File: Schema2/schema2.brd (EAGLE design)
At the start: 53 x 64.8 mm, 34 parts, among them IC1 LM2596S, IC2 78L05CPK, IC3 TL431ACDBZ, IC4 LM358D, X1 22-23-2021, X2 22-23-2021

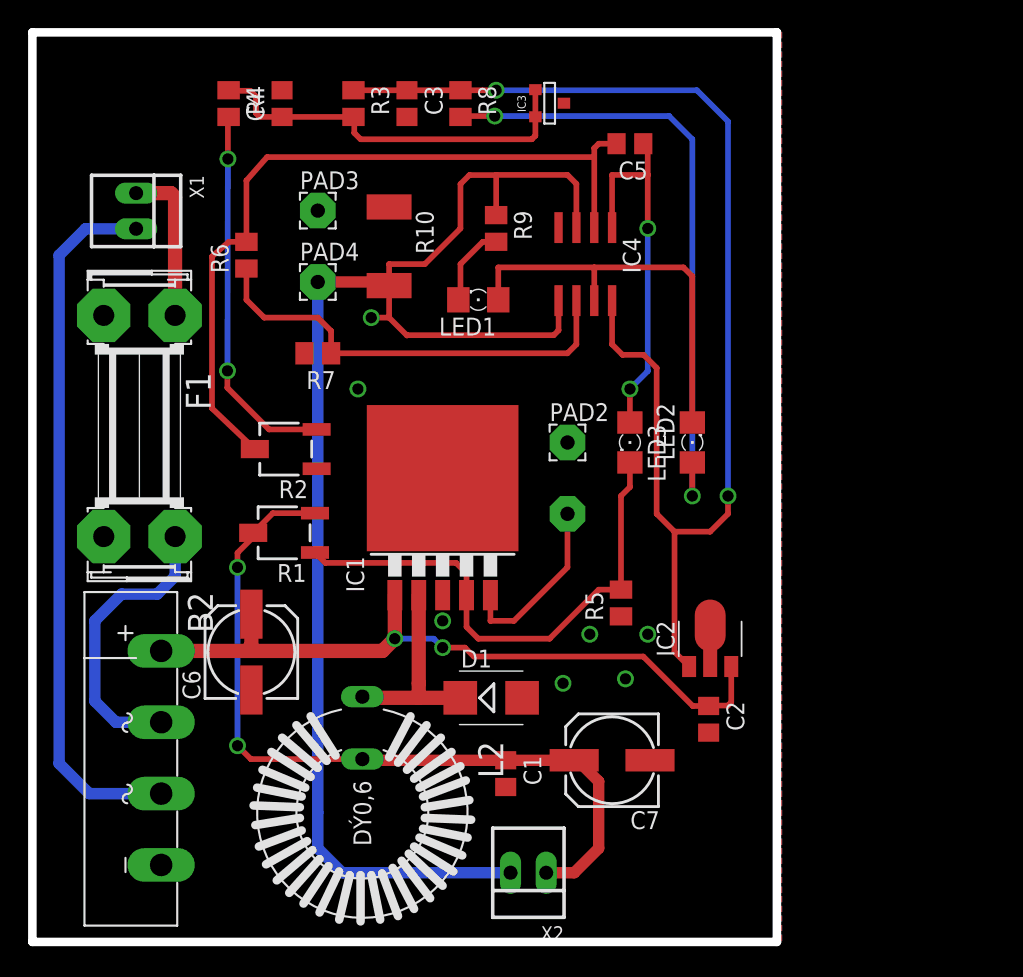
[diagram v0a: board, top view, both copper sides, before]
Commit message: update schema
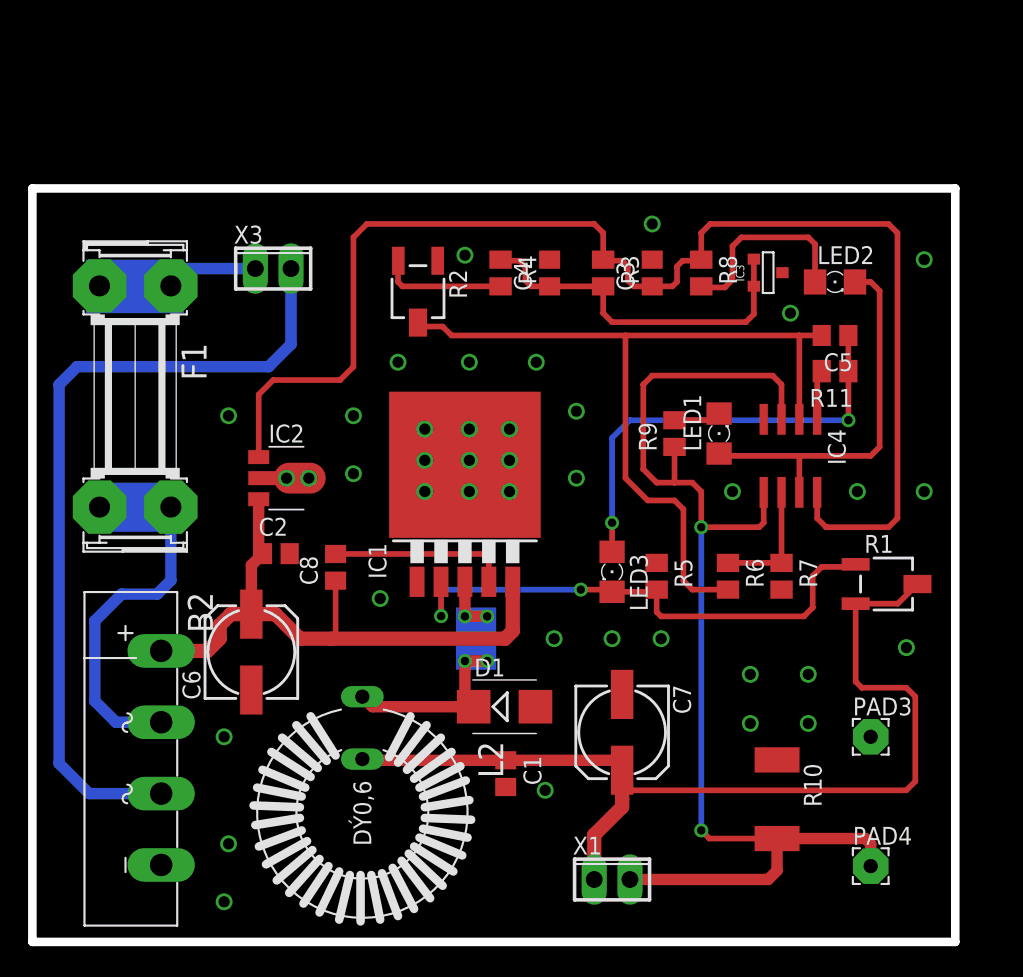
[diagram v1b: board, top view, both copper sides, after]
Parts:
- removed PAD1, PAD2: (no value), wirepad:2,54/1,0
- removed X2: 22-23-2021, con-molex:22-23-2021
- added C8: 1uF, eagle-ltspice:C0805
- added R11: 80R, resistor:M0805
- added X3: (no value), con-phoenix-254:2POL254
- IC1: value LM2596S -> XL4015; device linear:TO263-5 -> moje:TO263-5
- X1: value 22-23-2021 -> (none); device con-molex:22-23-2021 -> con-phoenix-254:2POL254
- moved X1 58.4 mm to (41.3, 4.45), turned to 0 degrees
- moved PAD4 57.3 mm to (59.7, 5.40)
- moved PAD3 54.3 mm to (59.7, 14.6)
- moved R10 48.1 mm to (53.0, 10.2)
- moved R1 43.0 mm to (60.8, 25.5), turned to 0 degrees
- moved R6 41.2 mm to (49.5, 26.0), turned to 270 degrees
- moved R7 36.6 mm to (53.3, 26.0), turned to 270 degrees
- moved C2 33.0 mm to (17.4, 27.6), turned to 0 degrees
- moved IC2 32.3 mm to (18.1, 33.0), turned to 270 degrees
- moved R4 22.8 mm to (33.3, 47.6)
- moved C4 22.5 mm to (36.8, 47.6)
- moved R3 21.5 mm to (40.6, 47.6)
- moved C3 21.2 mm to (44.1, 47.6), turned to 90 degrees
- moved R8 21.0 mm to (47.6, 47.6)
- moved C5 20.0 mm to (57.1, 43.2)
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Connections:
- removed net N$8: IC1.5, PAD1.1
- new net N$4: IC4.1, R11.2
- new net N$5: C8.2, IC1.4
- net GND: now also IC1.1; no longer IC1.3, PAD2.1
- net N$1: now also X3.1; no longer X1.1
- net N$10: now also IC1.3; no longer IC1.2
- net N$11: now also R11.1; no longer IC4.1
- net N$12: now also X1.1; no longer X2.1
- net N$14: now also IC1.2; no longer IC1.4
- net N$21: now also X1.2; no longer X2.2
- net N$3: now also X3.2; no longer X1.2
- net VCC_IN: now also C8.1, IC1.5; no longer IC1.1
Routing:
- net N$20: track 45.0 -> 13.9 mm, vias 2 -> 0
- net N$16: track 31.6 -> 8.83 mm
- net N$21: track 103.9 -> 84.1 mm, vias 1 -> 2
- net N$7: track 27.1 -> 8.95 mm, vias 2 -> 0
- net N$12: track 57.1 -> 70.6 mm, vias 2 -> 0
- net N$8: track 12.7 -> 0.00 mm
- net N$5: track 0.00 -> 12.6 mm
- net N$3: track 50.6 -> 58.2 mm
- net VCC_IN: track 51.5 -> 44.2 mm, vias 2 -> 0
- net N$6: track 89.1 -> 96.2 mm, vias 2 -> 0
- net N$10: track 14.3 -> 20.6 mm, vias 0 -> 4
- net N$1: track 11.3 -> 6.53 mm
- net N$11: track 26.8 -> 31.5 mm
- net N$4: track 0.00 -> 3.75 mm
- net N$9: track 55.1 -> 58.8 mm
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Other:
- board size 53 x 64.8 mm -> 65.7 x 53.6 mm

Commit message: update schema
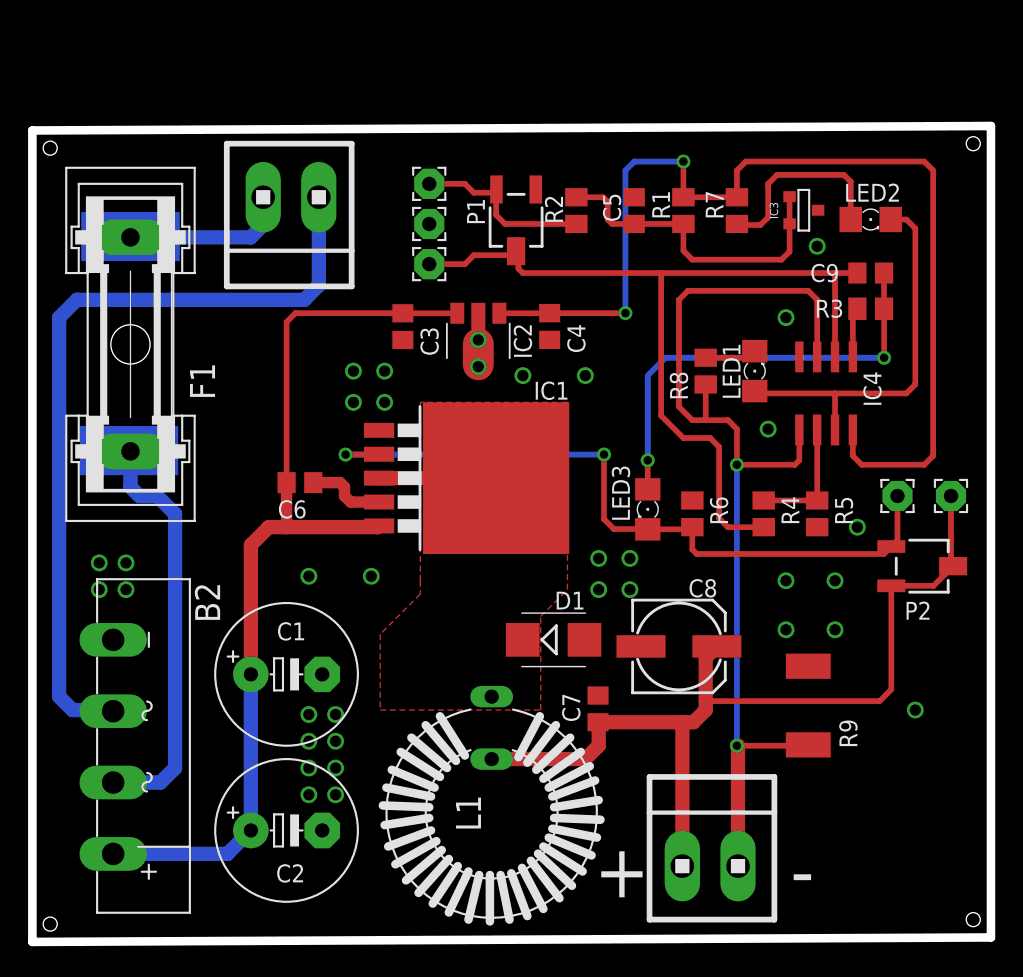
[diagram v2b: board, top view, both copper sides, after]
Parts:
- removed L2: 40uH, inductors:ED16
- removed R10: 0,05R, eagle-ltspice:R2512
- removed R11: 80R, resistor:M0805
- removed X1, X3: (no value), con-phoenix-254:2POL254
- added C9: 1uF, eagle-ltspice:C0805
- added J1, J2: (no value), con-amp:1X2MTA
- added L1: 40uH, inductors:ED16
- added P1, P2: 10K, pot:3223G
- added PAD2, PAD5, PAD6: (no value), wirepad:2,15/1,0
- C1, C2: value 10uF -> (none); device eagle-ltspice:C0805 -> adafruit:E5-10,5
- C3: value 1uF -> 10uF
- C6: value 470uF -> 1uF; device resistor:153CLV-0605 -> eagle-ltspice:C0805
- C7: value 470uF -> 10uF; device resistor:153CLV-0605 -> eagle-ltspice:C0805
- C8: value 1uF -> 470uF; device eagle-ltspice:C0805 -> resistor:153CLV-0605
- F1: value (none) -> FUSEGSH15; device fuse:SHK20Q -> fuse:GSH15
- IC2: value 78L05CPK -> 78L05
- IC3: value TL431ACDBZ -> TL431
- PAD3, PAD4: device wirepad:2,54/1,0 -> wirepad:2,15/1,0
- R1: value 10K -> 2,2K; device pot:3223G -> resistor:M0805
- R2: value 10K -> 68K; device pot:3223G -> resistor:M0805
- R3: value 2,2K -> 80R
- R4: value 71,5K -> 100K
- R5: value 270R -> 10K
- R6: value 90,9K -> 270R
- R7: value 10K -> 1K
- R9: value 1K -> 0,05R; device resistor:M0805 -> eagle-ltspice:R2512
- moved PAD4 57.9 mm to (28.3, 54.0)
- moved R1 30.3 mm to (46.4, 52.1), turned to 270 degrees
- moved R7 26.2 mm to (50.2, 52.1)
- moved R4 25.4 mm to (52.1, 30.5)
- moved C8 25.1 mm to (46.0, 21.0), turned to 0 degrees
- moved R9 21.6 mm to (55.2, 16.8), turned to 270 degrees
- moved C2 19.7 mm to (18.1, 7.94)
- moved R3 19.2 mm to (59.7, 45.1), turned to 180 degrees
- moved C3 18.2 mm to (26.4, 43.8), turned to 270 degrees
- moved PAD3 18.1 mm to (65.4, 31.8)
- moved C1 17.1 mm to (18.1, 19.1), turned to 0 degrees
- moved C5 16.8 mm to (42.9, 52.1), turned to 90 degrees
- moved IC2 16.8 mm to (31.8, 42.8), turned to 180 degrees
- moved R2 12.7 mm to (38.7, 52.1)
- moved C6 12.6 mm to (19.1, 32.7), turned to 0 degrees
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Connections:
- removed net N$6: C3.1, IC2.1, IC4.8, R3.1, R8.1
- new net VNN: C4.1, IC2.1, IC4.8, R1.1, R7.1
- net GND: now also C1.-, C2.-, C5.2, C7.2, C8.-, P1.1, PAD5.1, R5.2, R6.1, R9.1; no longer C1.2, C2.2, C6.-, C7.-, IC1.6, PAD3.1, R10.1, R2.1, R5.1, R7.2
- net N$1: now also F1.1, J1.1; no longer F1.1A, X3.1
- net N$10: now also IC1.6, L1.1; no longer L2.1
- net N$11: now also C9.1, R3.1; no longer C5.1, R11.1
- net N$12: now also C7.1, C8.+, J2.2, L1.2, P2.2, P2.3, PAD3.1; no longer C1.1, C7.+, L2.2, R1.2, R1.3, X1.1
- net N$14: now also P2.1, PAD2.1, R6.2; no longer R1.1, R5.2
- net N$15: now also C5.1, R1.2, R2.1; no longer C4.1, R3.2, R4.1
- net N$16: now also R4.1, R5.1; no longer R6.1, R7.1
- net N$18: now also R8.2; no longer R9.2
- net N$2: now also F1.2; no longer F1.2A
- net N$20: now also R7.2; no longer R8.2
- net N$21: now also J2.1, R8.1, R9.2; no longer PAD4.1, R10.2, R9.1, X1.2
- net N$3: now also J1.2; no longer X3.2
- net N$4: now also R3.2; no longer R11.2
- net N$5: now also C6.2; no longer C8.2
- net N$7: now also P1.3, PAD4.1, R2.2; no longer R2.3, R4.2
- net N$9: now also C9.2, P1.2, PAD6.1, R4.2; no longer C5.2, R2.2, R6.2
- net VCC_IN: now also C1.+, C2.+, C3.1, C6.1; no longer C2.1, C6.+, C8.1
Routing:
- net N$6: track 96.2 -> 0.00 mm
- net VNN: track 0.00 -> 74.7 mm, vias 0 -> 2
- net VCC_IN: track 44.2 -> 67.5 mm
- net N$14: track 38.4 -> 52.0 mm
- net N$10: track 20.6 -> 8.33 mm, vias 4 -> 0
- net N$21: track 84.1 -> 72.4 mm
- net N$5: track 12.6 -> 5.63 mm
- net N$2: track 22.9 -> 29.4 mm
- net N$12: track 70.6 -> 64.0 mm
- net N$1: track 6.53 -> 11.9 mm
- net N$7: track 8.95 -> 13.0 mm
- net N$9: track 58.8 -> 61.8 mm
- net N$15: track 25.7 -> 23.0 mm
- net N$3: track 58.2 -> 57.0 mm
- added copper zone on layer 1, net N$10
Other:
- board size 65.7 x 53.6 mm -> 68.2 x 58.1 mm
- board text added: "+"
- board text added: "-"
